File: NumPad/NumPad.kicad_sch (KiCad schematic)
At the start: 18 parts, among them J1 USB_C_Receptacle_USB2.0_16P, SW1 SW_Push, U1 ATmega32U4-A, Y1 16MHz

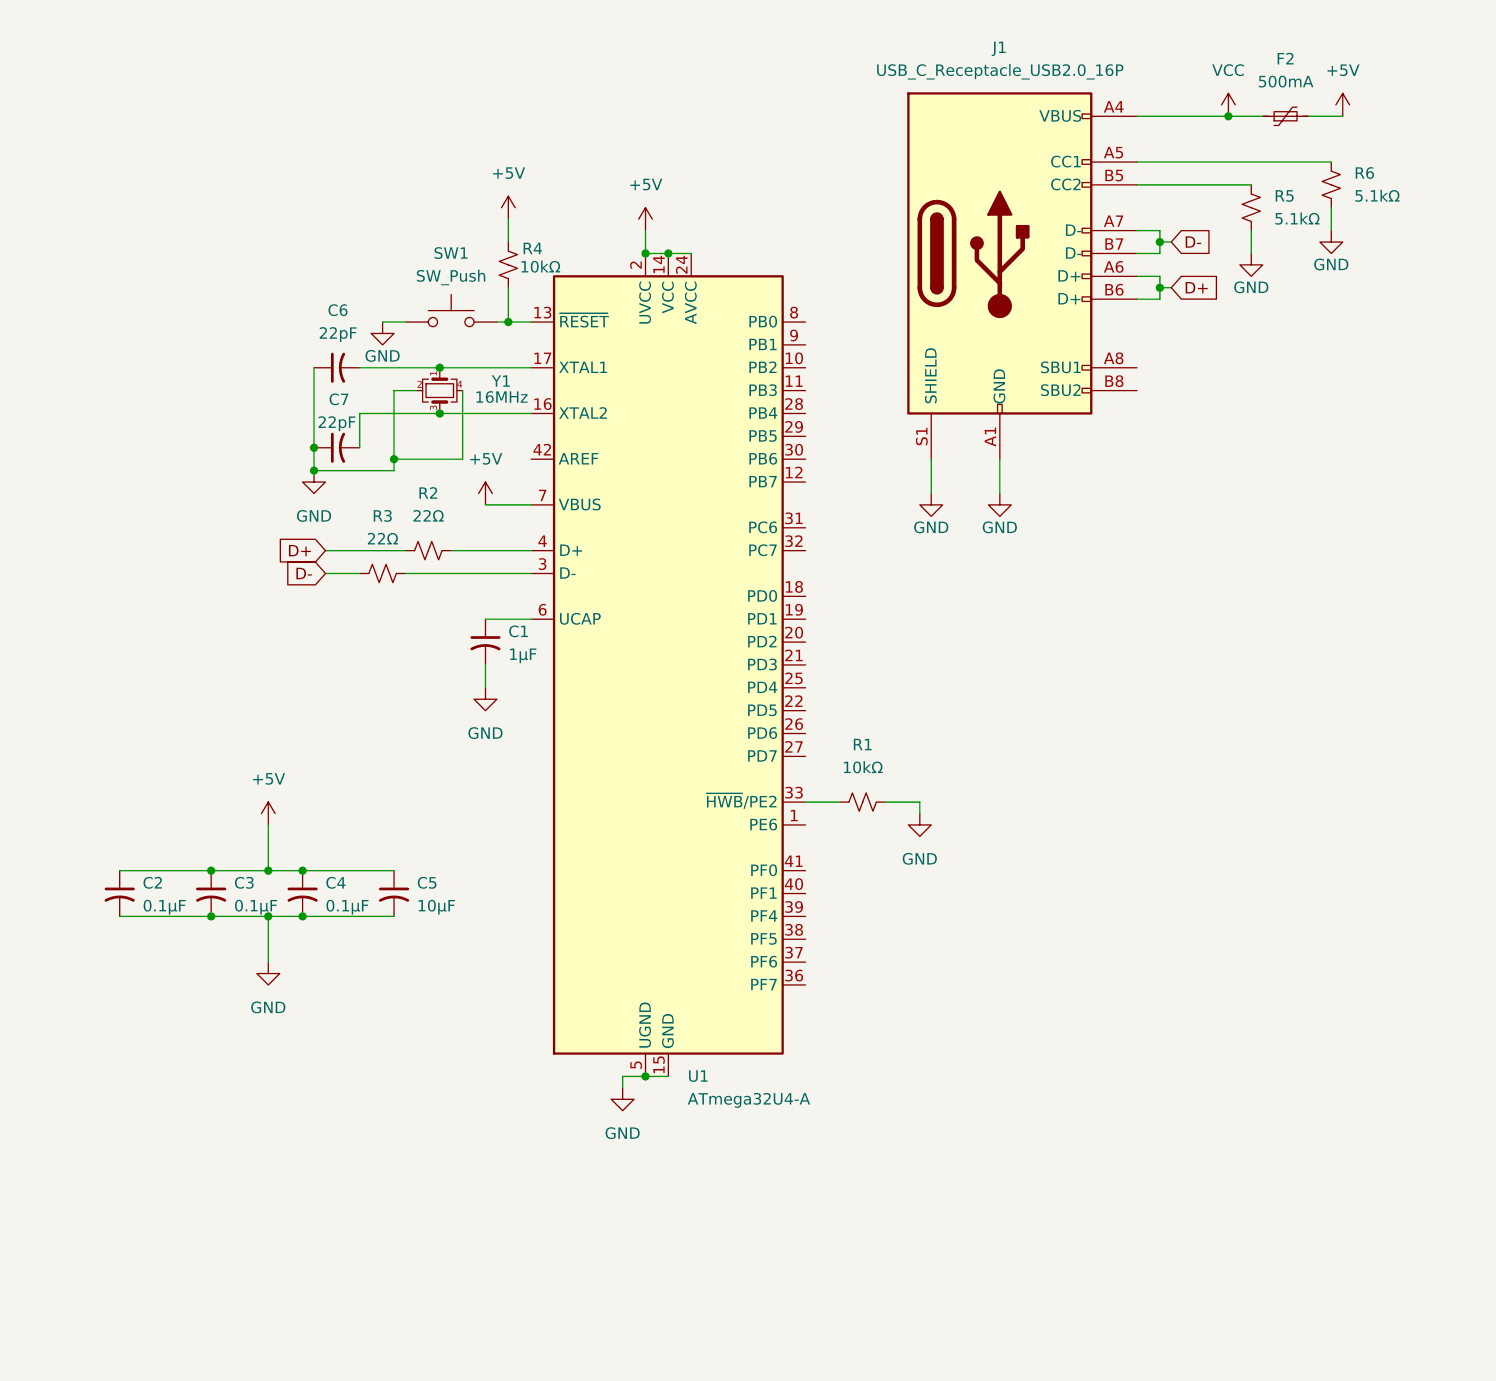
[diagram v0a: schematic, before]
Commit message: completed schematic V1
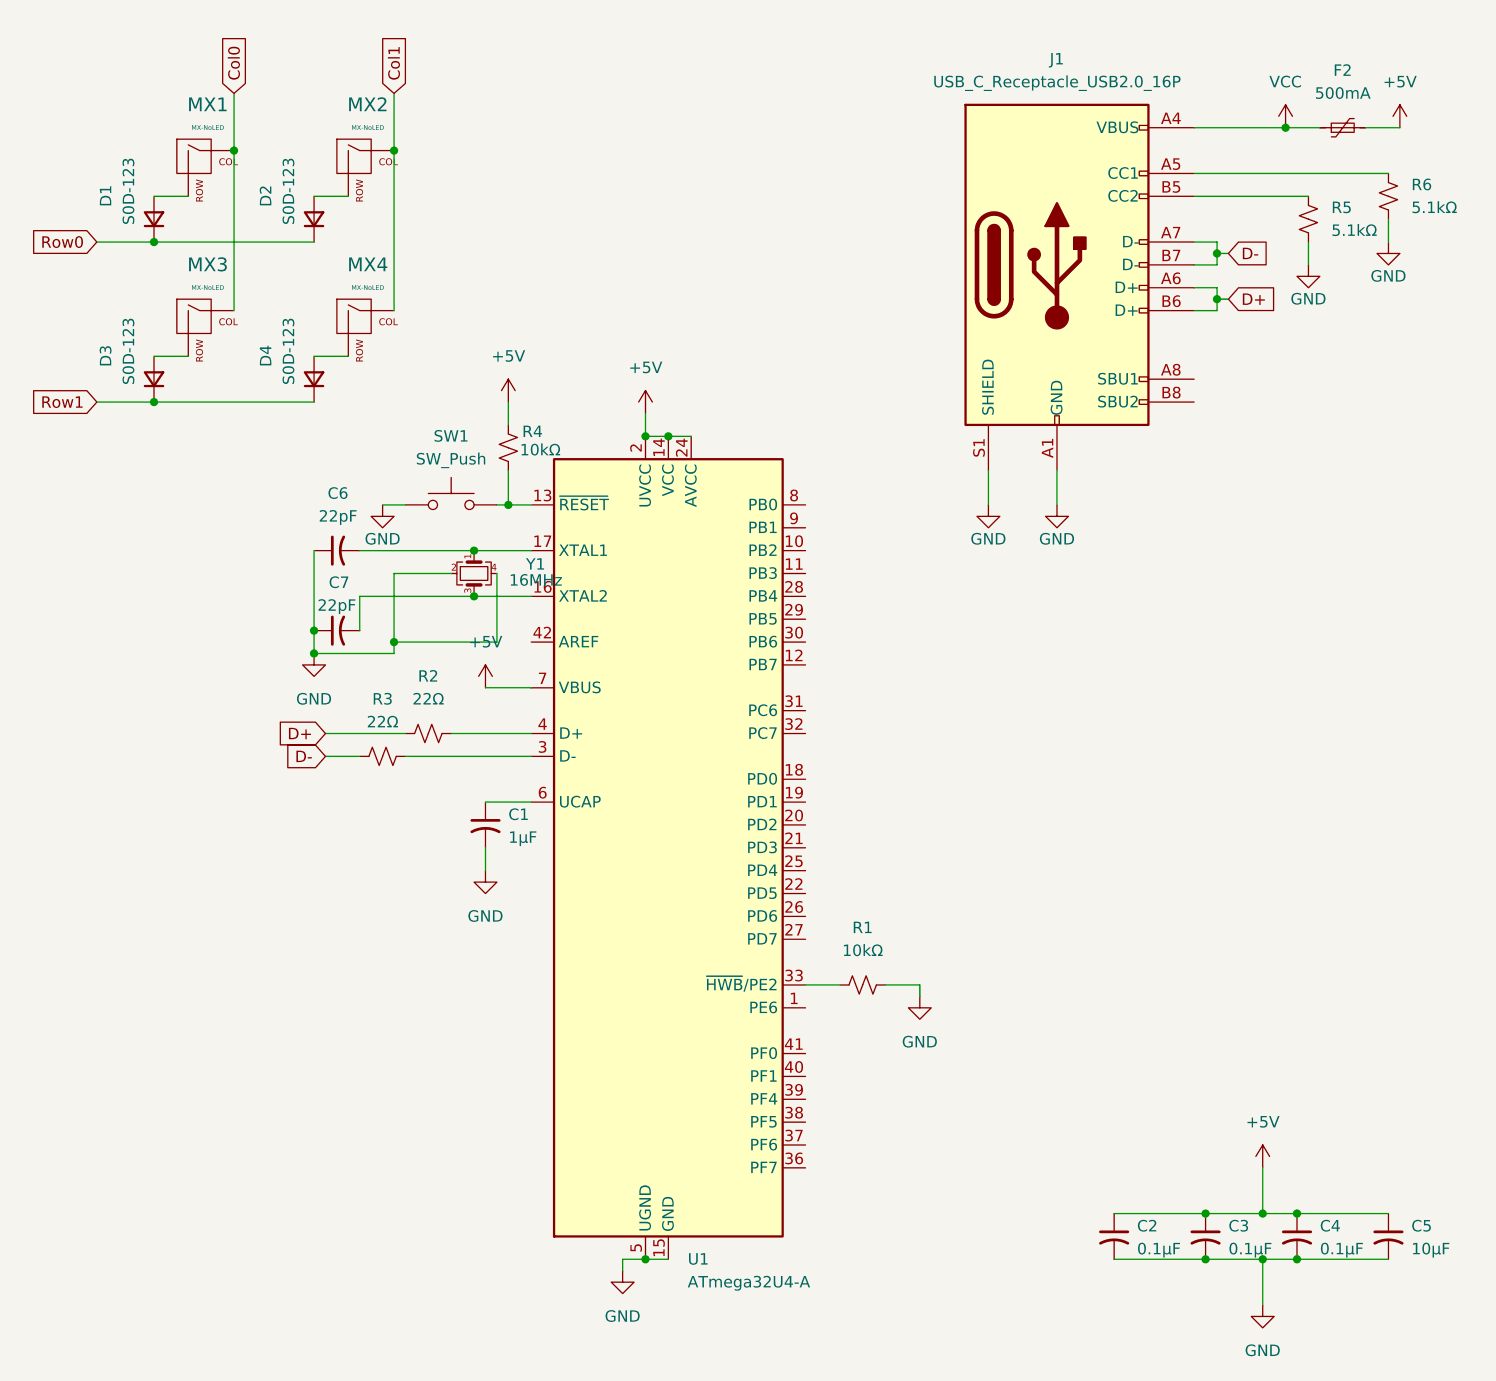
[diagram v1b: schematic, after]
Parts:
- added D1, D2, D3, D4: S0D-123, Diode_SMD:D_SOD-123, symbol Device:D_Small
- added MX1, MX2, MX3, MX4: MX-NoLED, MX_Alps_Hybrid:MX-1U, symbol MX_Alps_Hybrid:MX-NoLED
- C1, C2, C3, C4, C5, C6, C7: footprint (none) -> Capacitor_SMD:C_0805_2012Metric
- F2: footprint (none) -> Fuse:Fuse_1206_3216Metric
- J1: footprint (none) -> Connector_USB:USB_C_Receptacle_HRO_TYPE-C-31-M-12
- R1, R2, R3, R4, R5, R6: footprint (none) -> Resistor_SMD:R_0805_2012Metric
- SW1: footprint (none) -> random-keyboard-parts:SKQG-1155865
- Y1: footprint (none) -> Crystal:Crystal_SMD_3225-4Pin_3.2x2.5mm
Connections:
- new net: D1.2 (A), MX1.2 (ROW)
- new net: D4.2 (A), MX4.2 (ROW)
- new net: D3.2 (A), MX3.2 (ROW)
- new net: D2.2 (A), MX2.2 (ROW)
- new net Col0: MX1.1 (COL), MX3.1 (COL)
- new net Col1: MX2.1 (COL), MX4.1 (COL)
- new net Row0: D1.1 (K), D2.1 (K)
- new net Row1: D3.1 (K), D4.1 (K)
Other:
- moved on the sheet: C1, C2, C3, C4, C5, C6, C7, F2, J1, R1, R2, R3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
